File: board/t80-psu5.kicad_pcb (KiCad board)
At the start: 2 copper layers, 26 x 80 mm, 18 parts, among them J1 Conn_01x02_Female, U2 FR8205

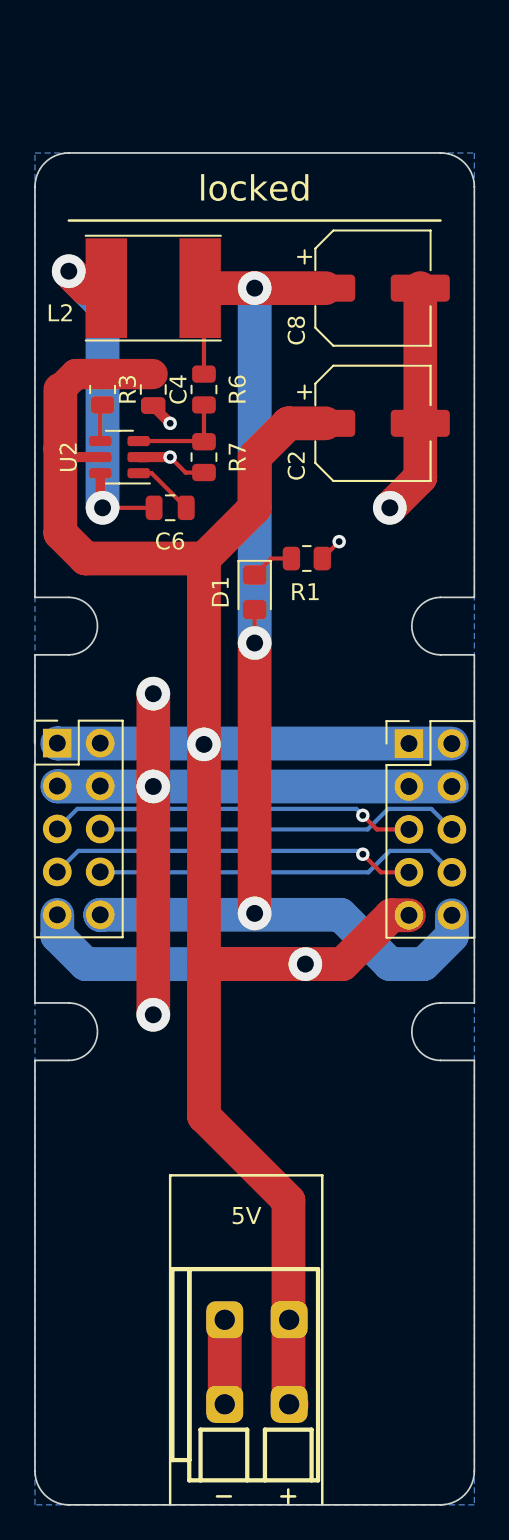
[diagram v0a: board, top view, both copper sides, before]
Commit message: WIP
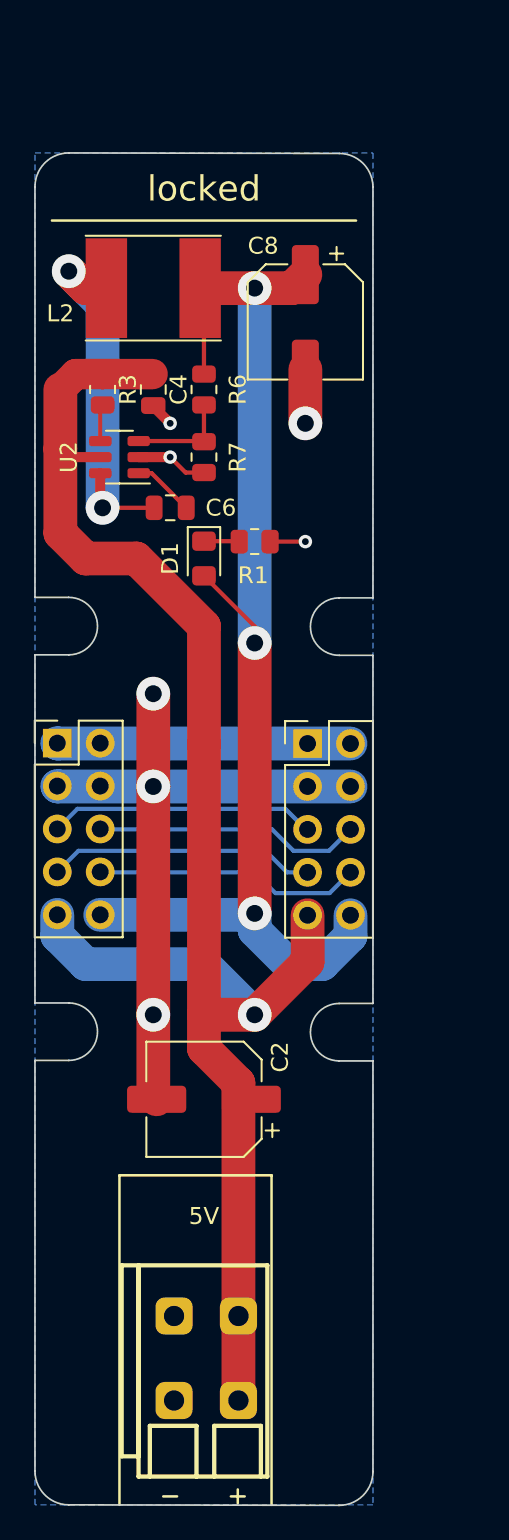
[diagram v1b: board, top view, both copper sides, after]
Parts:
- moved C2 41.2 mm to (95.0, 116.0), turned to 180 degrees
- moved X2 6.00 mm to (101.1, 95.0)
- moved C8 4.47 mm to (101.0, 70.0), turned to -90 degrees
- moved NT2 4.24 mm to (98.0, 111.0)
- moved D1 3.61 mm to (95.0, 84.0)
- moved R1 3.25 mm to (98.0, 83.0)
- moved J1 3.01 mm to (93.2, 128.8)
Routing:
- net +5V: track 96.5 -> 77.4 mm, vias 1 -> 0
- net GND: track 44.4 -> 35.1 mm
- net /IRQ: track 21.9 -> 15.8 mm
- net /SCL: track 21.8 -> 15.8 mm, vias 1 -> 0
- net /PWR_LINE_GND: track 23.4 -> 17.4 mm
- net /PWR_LINE_12V: track 23.4 -> 17.4 mm
- net /RST: track 21.9 -> 15.9 mm, vias 1 -> 0
- net /SDA: track 21.8 -> 15.9 mm
- net /PWR_LINE_3V3: track 24.0 -> 18.6 mm
- net +3V3: track 51.6 -> 54.0 mm
- net /PWR_LINE_5V: track 23.9 -> 22.0 mm
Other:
- board size 26 x 80 mm -> 20 x 80 mm

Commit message: WIP
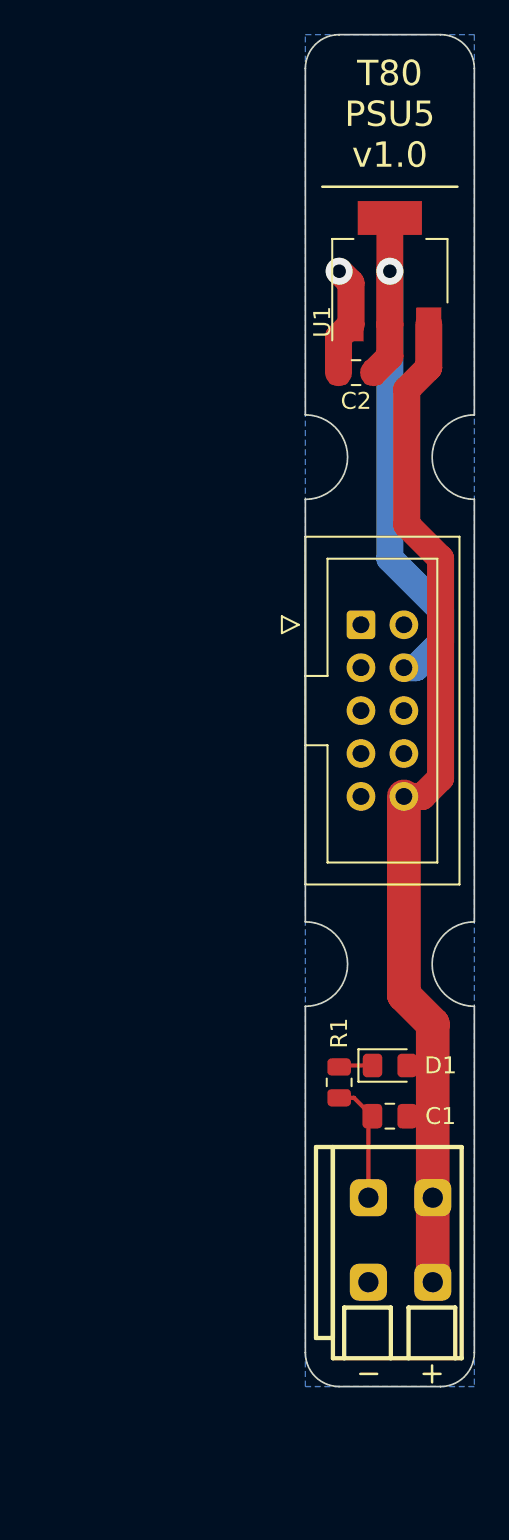
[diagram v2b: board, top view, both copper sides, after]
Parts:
- removed C4, C6: 100n, Capacitor_SMD:C_0805_2012Metric
- removed C8: 100u/12V, Capacitor_SMD:CP_Elec_6.3x5.4
- removed L2: 6.8uH, Drake:CKCS6028
- removed NT2, NT3, NT4, NT5: NetTie_2, t80:NetTie-2mm-T80
- removed R3: 100k, Resistor_SMD:R_0805_2012Metric
- removed R6: 30k 1%, Resistor_SMD:R_0805_2012Metric
- removed R7: 6.65k 1%, Resistor_SMD:R_0805_2012Metric
- removed U2: FR8205, Package_TO_SOT_SMD:SOT-23-6
- removed X1, X2: ~, Connector_PinHeader_2.54mm:PinHeader_2x05_P2.54mm_Vertical
- added C1: 10u, Capacitor_SMD:C_0805_2012Metric_Pad1.18x1.45mm_HandSolder, F.Cu at (106.0, 117.0)
- added U1: LM1117-3.3, Package_TO_SOT_SMD:SOT-223-3_TabPin2, F.Cu at (106.0, 67.0)
- added X3: ~, Connector_IDC:IDC-Header_2x05_P2.54mm_Vertical, F.Cu at (104.3, 87.9)
- C2: value 100u/12V -> 10u; footprint Capacitor_SMD:CP_Elec_6.3x5.4 -> Capacitor_SMD:C_0805_2012Metric_Pad1.18x1.45mm_HandSolder
- moved C2 43.9 mm to (104.0, 73.0)
- moved R1 32.4 mm to (103.0, 115.0), turned to -90 degrees
- moved D1 32.0 mm to (106.0, 114.0), turned to 0 degrees
- moved J1 13.5 mm to (104.7, 121.8)
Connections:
- C2 pad 1: +5V -> +3V3
- D1 pad 2: +3V3 -> +5V
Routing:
- net Net-(U2-LX): track 22.6 -> 0.00 mm, vias 2 -> 0
- net /PWR_LINE_5V: track 22.0 -> 0.00 mm, vias 1 -> 0
- net GND: track 35.1 -> 13.9 mm, vias 6 -> 1
- net /PWR_LINE_3V3: track 18.6 -> 0.00 mm
- net +3V3: track 54.0 -> 35.6 mm, vias 3 -> 1
- net /PWR_LINE_12V: track 17.4 -> 0.00 mm
- net /PWR_LINE_GND: track 17.4 -> 0.00 mm, vias 1 -> 0
- net +5V: track 77.4 -> 60.3 mm
- net /SDA: track 15.9 -> 0.00 mm
- net /RST: track 15.9 -> 0.00 mm
- net /IRQ: track 15.8 -> 0.00 mm
- net /SCL: track 15.8 -> 0.00 mm
- net Net-(U2-FB): track 6.05 -> 0.00 mm
- net Net-(U2-BST): track 3.66 -> 0.00 mm
- net Net-(U2-SHDN): track 2.19 -> 0.00 mm
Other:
- board size 20 x 80 mm -> 10 x 80 mm
- board text added: "T80 PSU5 v1.0"
- board text removed: "5V"
- board text removed: "locked"
